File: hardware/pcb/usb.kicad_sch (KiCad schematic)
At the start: 0 parts

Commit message: usb power
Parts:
- added D1, D2, D3: ESD441, ESD441DPLR:ESD441DPLR, symbol Device:D_Small
- added J1: USB_C_Receptacle_USB2.0_14P, PCM_ckl-connector:USB_C_Receptacle_HRO_TYPE-C-31-M-12, symbol Connector:USB_C_Receptacle_USB2.0_14P
- added U5: ECMF02-2AMX6, Package_DFN_QFN:ST_UQFN-6L_1.5x1.7mm_P0.5mm, symbol Power_Protection:ECMF02-2AMX6
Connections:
- new net CC1: D1.1 (K), J1.A5 (CC1)
- new net CC2: D2.1 (K), J1.B5 (CC2)
- new net D+: U5.6 (D+_out)
- new net D-: U5.5 (D-_out)
- new net DIRTY_D+: J1.A6 (D+), J1.B6 (D+), U5.1 (D+_in)
- new net DIRTY_D-: J1.A7 (D-), J1.B7 (D-), U5.2 (D-_in)
- new net GND: D1.2 (A), D2.2 (A), D3.2 (A), J1.A1 (GND), J1.A12 (GND), J1.B1 (GND), J1.B12 (GND), J1.SH (SHIELD), U5.3 (GND)
- new net VBUS: D3.1 (K), J1.A4 (VBUS), J1.A9 (VBUS), J1.B4 (VBUS), J1.B9 (VBUS)

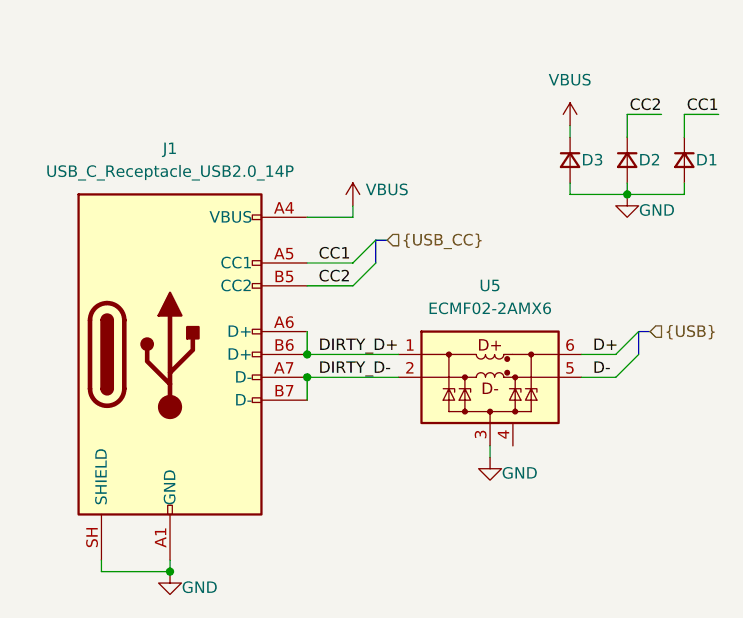
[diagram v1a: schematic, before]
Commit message: finished power
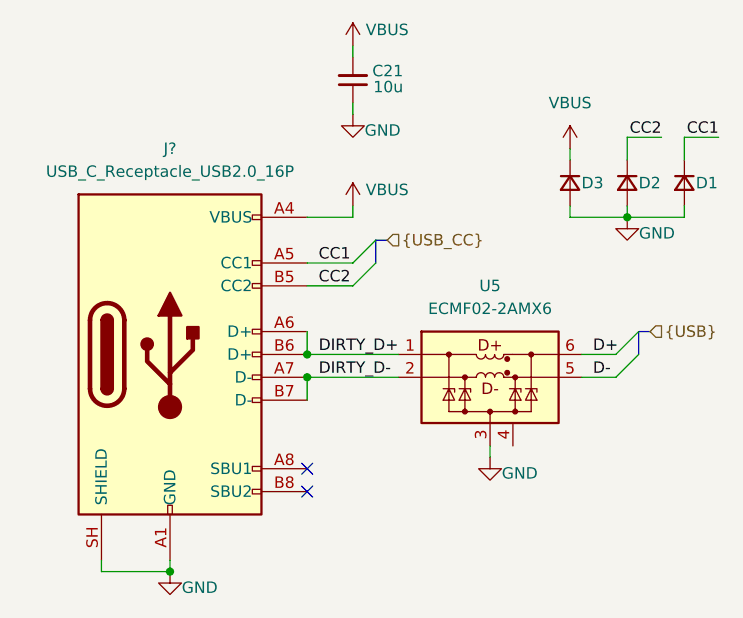
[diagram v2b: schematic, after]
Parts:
- removed J1: USB_C_Receptacle_USB2.0_14P, PCM_ckl-connector:USB_C_Receptacle_HRO_TYPE-C-31-M-12, symbol Connector:USB_C_Receptacle_USB2.0_14P
- added C21: 10u, symbol Device:C_Small
- added J?: USB_C_Receptacle_USB2.0_16P, symbol Connector:USB_C_Receptacle_USB2.0_16P
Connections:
- net CC1: now also J?.A5 (CC1)
- net CC2: now also J?.B5 (CC2)
- net DIRTY_D+: now also J?.A6 (D+), J?.B6 (D+)
- net DIRTY_D-: now also J?.A7 (D-), J?.B7 (D-)
- net GND: now also C21.1, J?.A1 (GND), J?.A12 (GND), J?.B1 (GND), J?.B12 (GND), J?.SH (SHIELD)
- net VBUS: now also C21.2, J?.A4 (VBUS), J?.A9 (VBUS), J?.B4 (VBUS), J?.B9 (VBUS)
- no-connect marks 0 -> 2
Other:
- moved on the sheet: D1, D2, D3
